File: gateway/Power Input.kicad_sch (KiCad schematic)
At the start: 12 parts, among them IC701 INA219AxD, X701 7-16 V

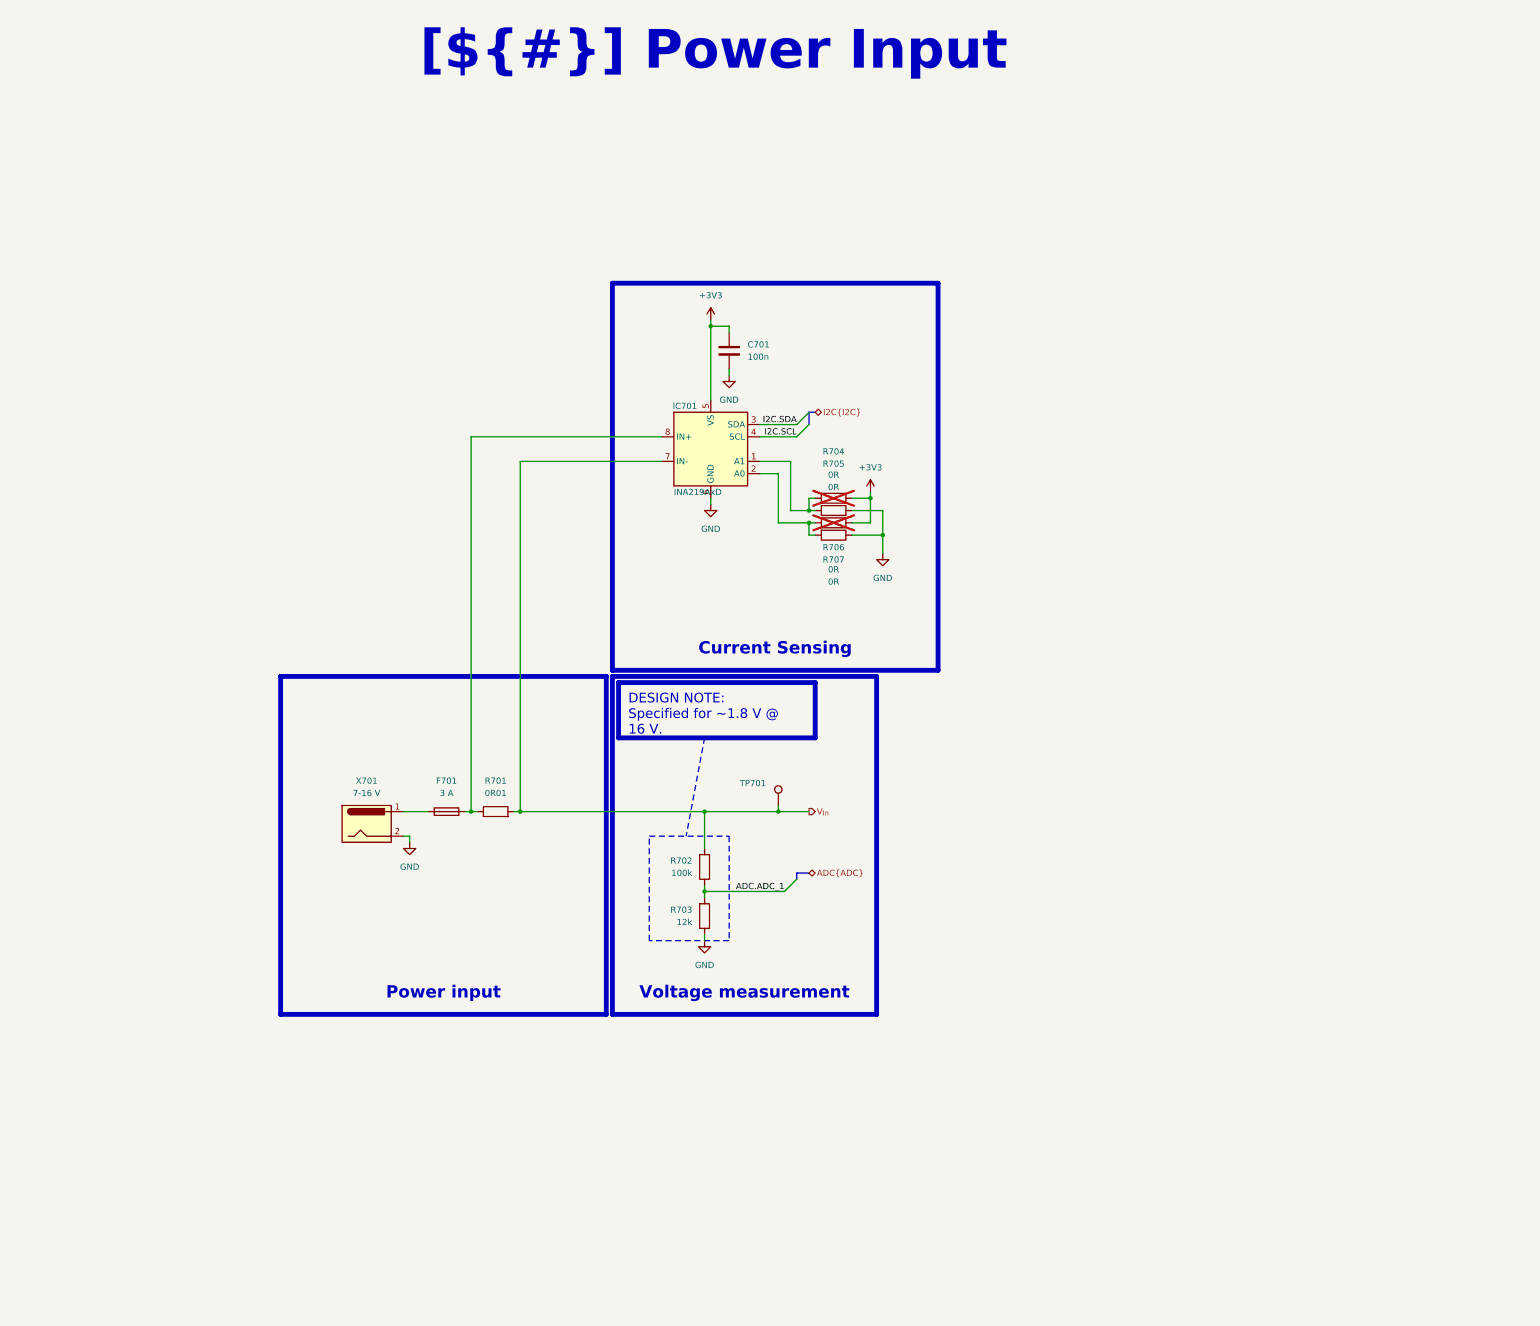
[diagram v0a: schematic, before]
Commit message: Working on PCB
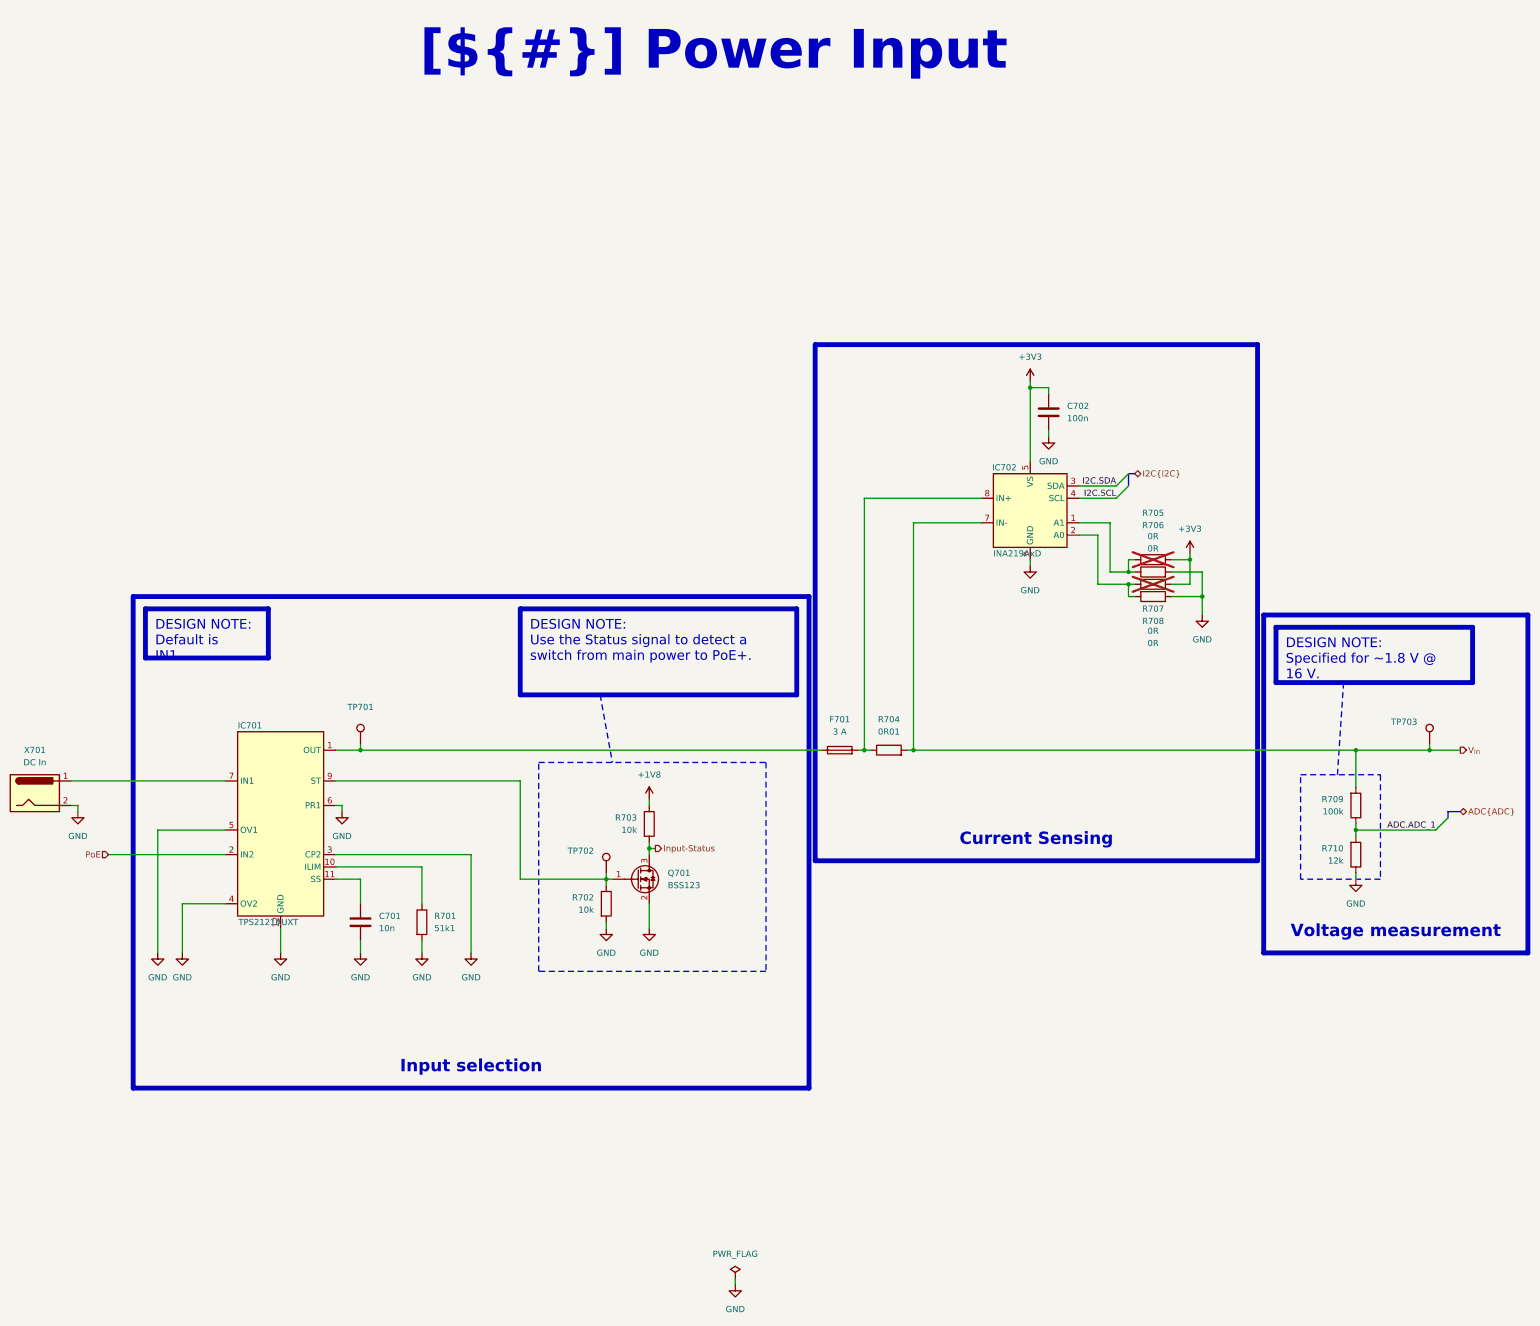
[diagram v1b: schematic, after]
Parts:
- added C701: 10n, Capacitor_SMD:C_0805_2012Metric, symbol Device:C
- added IC701: TPS2121RUXT, Texas Instruments:RUX0012A, symbol Texas Instruments:TPS2121RUXT
- added Q701: BSS123, Package_TO_SOT_SMD:SOT-23, symbol Transistor_FET:BSS123
- added R701: 51k1, Resistor_SMD:R_0805_2012Metric, symbol Device:R
- added R702, R703: 10k, Resistor_SMD:R_0805_2012Metric, symbol Device:R
- added TP701, TP702: ~, Testpoints_Kampi:TestPoint_Pad_1.0x1.0mm, symbol Connector:TestPoint
- TP703: renamed from TP701; value (none) -> ~
- X701: value 7-16 V -> DC In
- renumbered C701 to C702, IC701 to IC702, R701 to R704, R704 to R705, R705 to R706, R706 to R707, R707 to R708, R702 to R709, R703 to R710
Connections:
- net GND: now also C701.2, IC701.12 (GND), IC701.3 (CP2), IC701.4 (OV2), IC701.5 (OV1), IC701.6 (PR1), Q701.2 (S), R701.2, R702.2
- net at X701.1: now also IC701.7 (IN1); no longer F701.1
- new net: IC701.9 (ST), Q701.1 (G), R702.1, TP702.1
- new net: IC701.10 (ILIM), R701.1
- new net: C701.1, IC701.11 (SS)
- new net: F701.1, IC701.1 (OUT), IC701.8 (OUT), TP701.1
- new net +1V8: R703.1
- new net Input-Status: Q701.3 (D), R703.2
- new net PoE: IC701.2 (IN2)
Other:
- moved on the sheet: C702, F701, IC702, R704, R705, R706, R707, R708, R709, R710, TP703, X701
